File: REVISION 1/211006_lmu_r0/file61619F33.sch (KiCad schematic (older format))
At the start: 36 parts

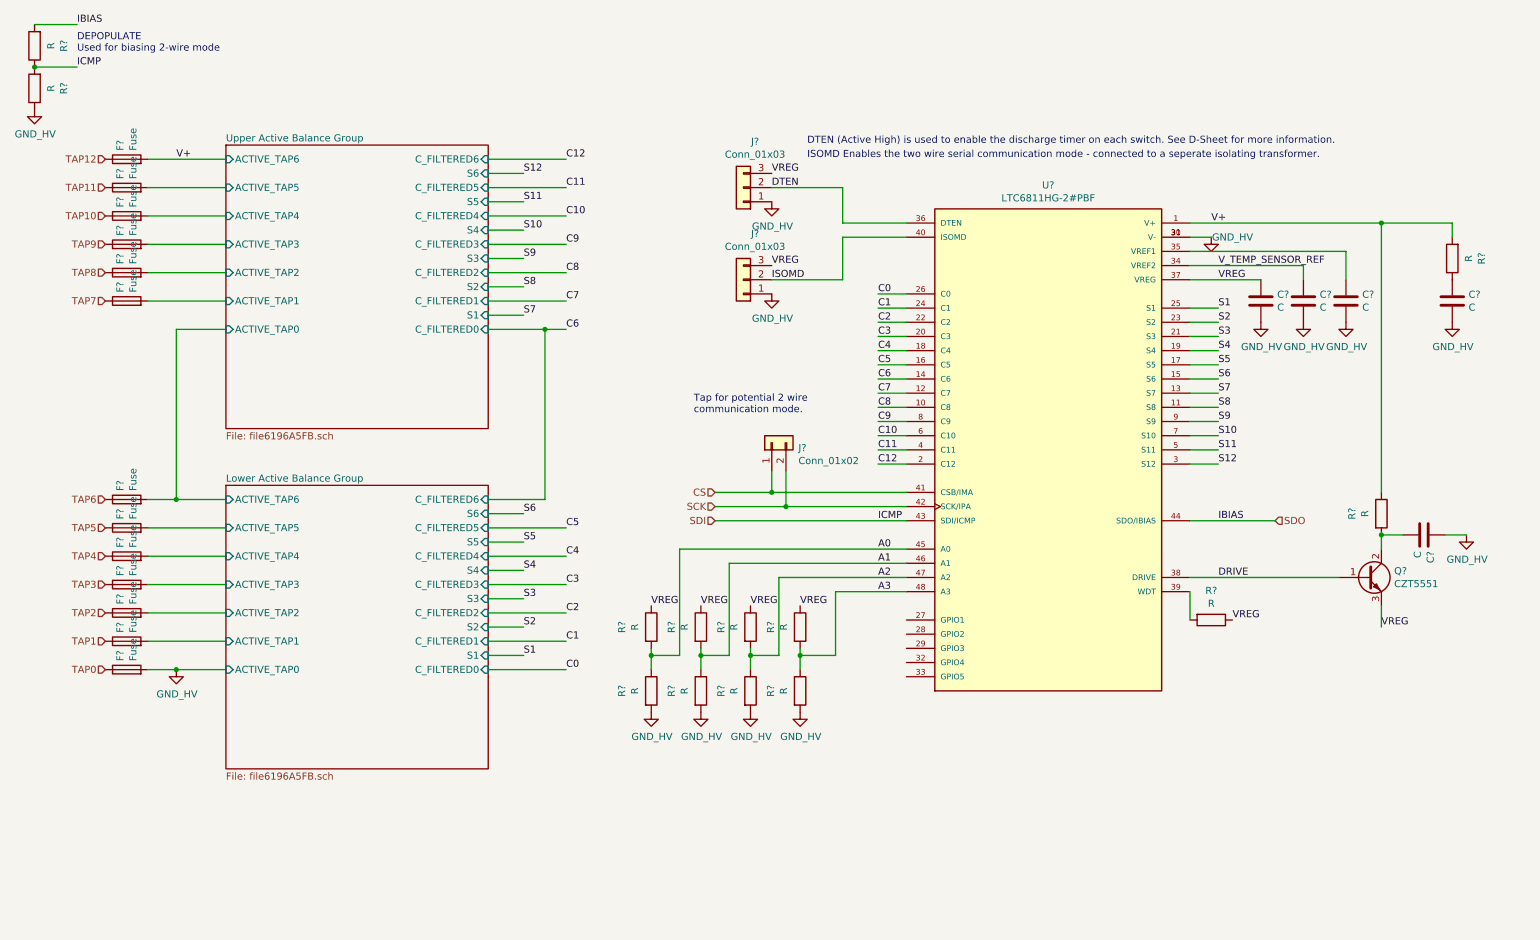
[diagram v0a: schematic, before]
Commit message: Finished schematic, ready for pcb layout
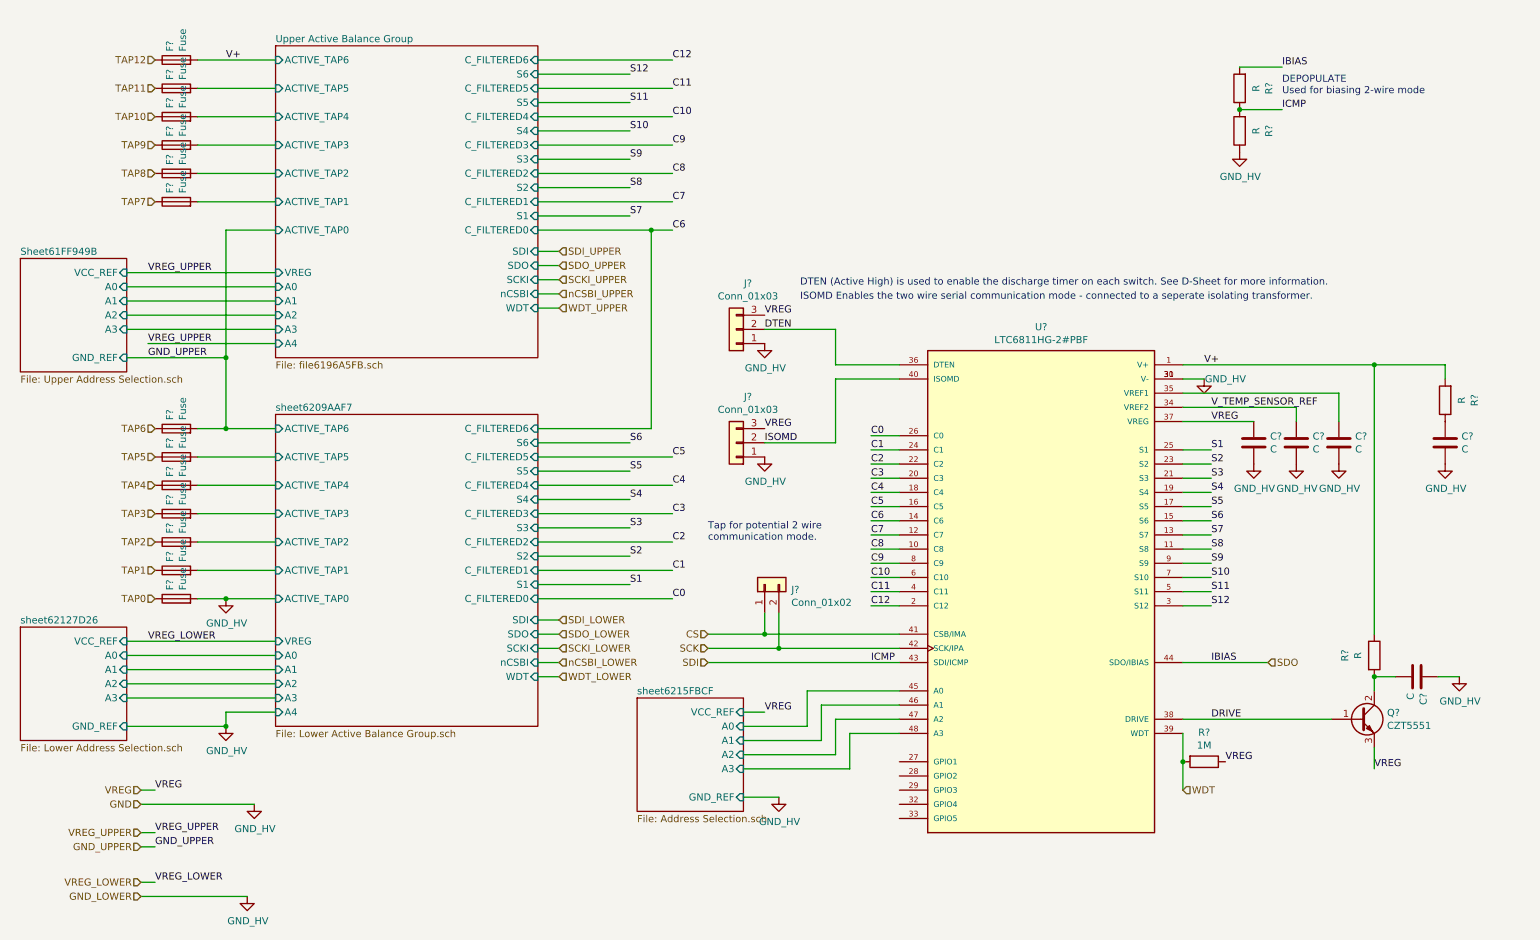
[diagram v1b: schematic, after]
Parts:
- removed R? (x8): R, symbol Device:R
- R?: value R -> 1M
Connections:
- net WDT: now reaches R?.2, U?.39 (WDT)
- net A0 renamed sheet6215FBCF/A0
- net A1 renamed sheet6215FBCF/A1
- net A2 renamed sheet6215FBCF/A2
- net A3 renamed sheet6215FBCF/A3
- net Lower Active Balance Group/ACTIVE_TAP1 renamed sheet6209AAF7/ACTIVE_TAP1
- net Lower Active Balance Group/ACTIVE_TAP2 renamed sheet6209AAF7/ACTIVE_TAP2
- net Lower Active Balance Group/ACTIVE_TAP3 renamed sheet6209AAF7/ACTIVE_TAP3
- net Lower Active Balance Group/ACTIVE_TAP4 renamed sheet6209AAF7/ACTIVE_TAP4
- net Lower Active Balance Group/ACTIVE_TAP5 renamed sheet6209AAF7/ACTIVE_TAP5
- net Lower Active Balance Group/ACTIVE_TAP6 renamed GND_UPPER
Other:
- moved on the sheet: C?, F?, J?, Q?, R?, U?
